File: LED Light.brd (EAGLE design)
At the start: 78.7 x 78.7 mm, 9 parts, among them J1 AVR_SPI_PRG_6NS, U1 Tiny85-20-SMT

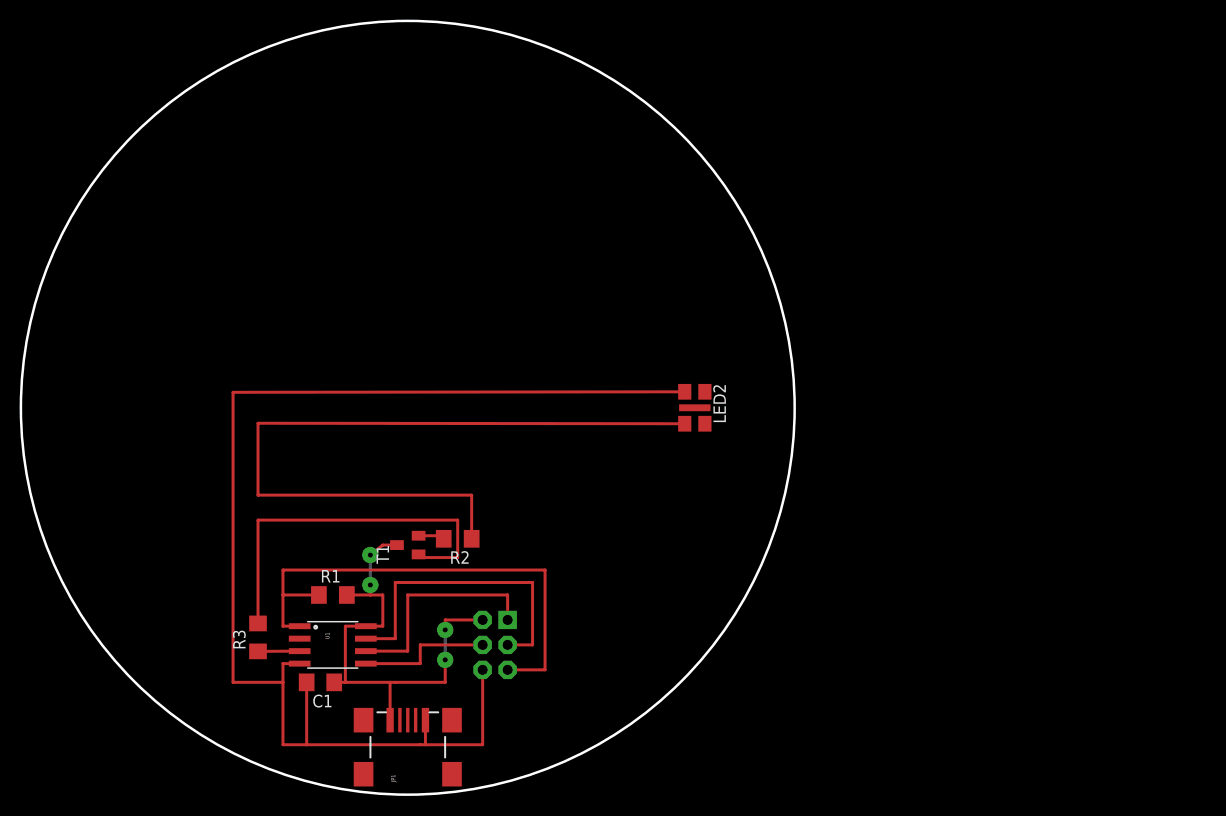
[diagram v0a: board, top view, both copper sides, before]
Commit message: Night-light lamp, including PNGs for milling and PDFs for laser-cutting.
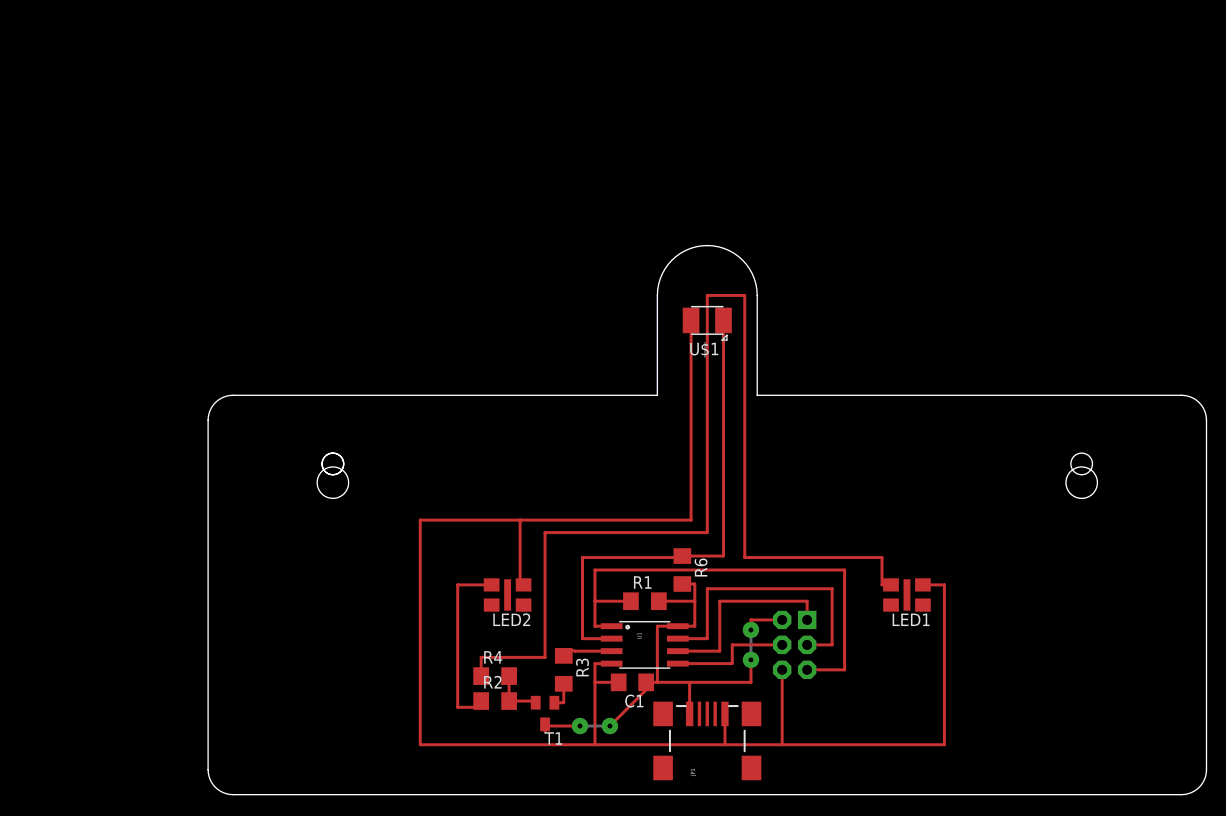
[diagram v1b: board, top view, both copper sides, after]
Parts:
- added LED1: ML-EFAB, LED Light:ML-E-FAB
- added R4: (no value), rcl:R1206
- added R6: 49.9K, rcl:R1206
- added U$1: PHOTOTRANSISTOR-NPN-OP580AD, LED Light:OP580DA
- moved R1 31.8 mm to (44.5, 19.7)
- moved U1 31.8 mm to (44.5, 15.2)
- moved C1 31.8 mm to (43.2, 11.4)
- moved R3 31.3 mm to (36.2, 12.7), turned to 270 degrees
- moved JP1 30.5 mm to (50.8, 4.45)
- moved J1 30.5 mm to (59.7, 15.2)
- moved LED2 26.9 mm to (30.5, 20.3), turned to 180 degrees
- moved T1 22.1 mm to (34.3, 8.26), turned to 180 degrees
- moved R2 16.9 mm to (29.2, 9.53), turned to 0 degrees
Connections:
- new net N$5: LED1.A@1, R4.1
- new net N$7: R6.1, U$1.COLLECTOR, U1.2
- net GND: now also LED1.C@1, U$1.EMITTER
- net N$1: now also R4.2
- net VCC: now also R6.2
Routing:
- net N$5: track 0.00 -> 109.9 mm
- net N$3: track 76.9 -> 18.9 mm
- net N$7: track 0.00 -> 49.7 mm
- net GND: track 127.3 -> 172.6 mm
- net N$2: track 38.9 -> 2.88 mm
- net VCC: track 48.8 -> 55.7 mm
- net N$1: track 2.69 -> 5.42 mm
- net SCK: track 31.6 -> 29.0 mm
- net MISO: track 22.7 -> 20.1 mm
- net RESET: track 51.7 -> 50.4 mm
- net MOSI: track 13.8 -> 12.5 mm
- net N$4: track 4.24 -> 4.98 mm
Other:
- board size 78.7 x 78.7 mm -> 101.6 x 55.9 mm
